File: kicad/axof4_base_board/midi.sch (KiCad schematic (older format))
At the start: 9 parts, among them J4 MIDI_IN, J5 MIDI_OUT, U8 6N137

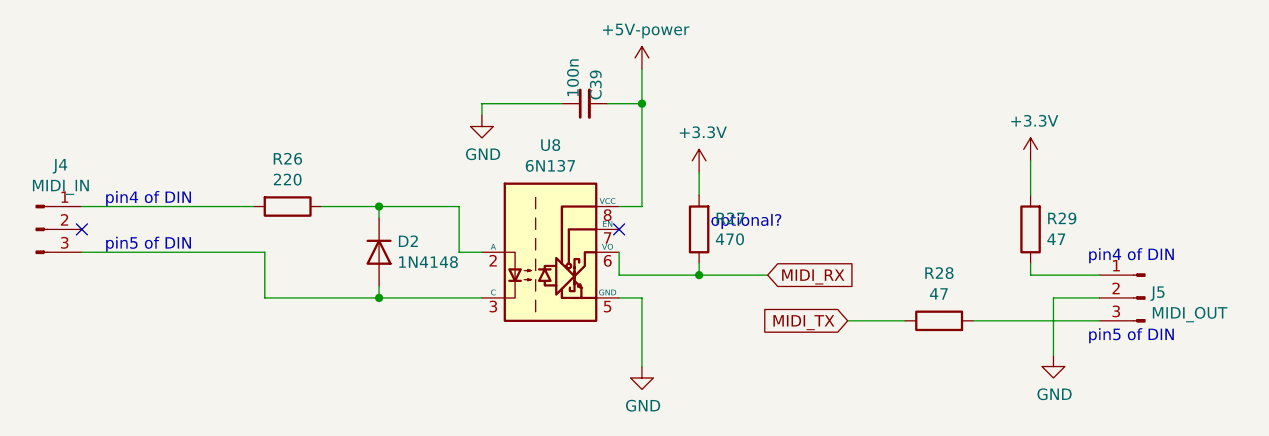
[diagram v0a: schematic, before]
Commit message: cleanup, dedicated PCB WIP
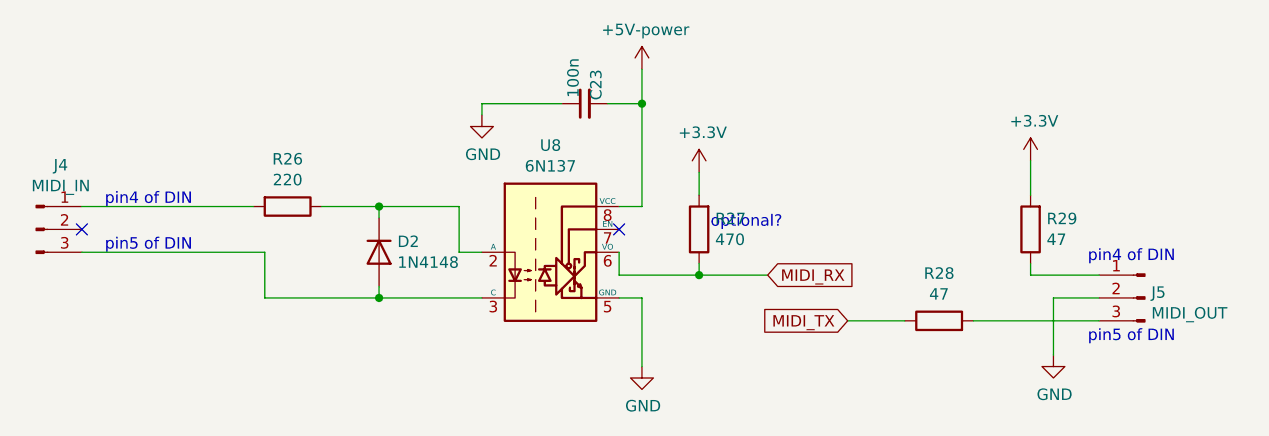
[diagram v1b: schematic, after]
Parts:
- J4, J5: footprint (none) -> Connector_PinHeader_2.54mm:PinHeader_1x03_P2.54mm_Vertical
- R26, R27, R28, R29: footprint (none) -> Resistor_SMD:R_1206_3216Metric_Pad1.42x1.75mm_HandSolder
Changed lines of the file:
@@
 $Descr A4 11693 8268
 encoding utf-8
-Sheet 6 6
+Sheet 6 7
 Title ""
 Date ""
@@
 AR Path="/5ED86ED4/5ECDCA2B" Ref="#PWR?"  Part="1"
 AR Path="/5EE2DB57/5ECDCA2B" Ref="#PWR037"  Part="1"
-F 0 "#PWR037" H 7800 3150 50  0001 C CNN
+AR Path="/5F736ED6/5ECDCA2B" Ref="#PWR?"  Part="1"
+F 0 "#PWR?" H 7800 3150 50  0001 C CNN
 F 1 "+3.3V" H 7815 3473 50  0000 C CNN
 F 2 "" H 7800 3300 50  0001 C CNN
@@
 AR Path="/5ED86ED4/5ECE0CFC" Ref="C?"  Part="1"
 AR Path="/5EE2DB57/5ECE0CFC" Ref="C39"  Part="1"
-F 0 "C39" H 6000 3000 50  0000 R CNN
+AR Path="/5F736ED6/5ECE0CFC" Ref="C?"  Part="1"
+F 0 "C?" H 6000 3000 50  0000 R CNN
 F 1 "100n" H 6050 3100 50  0000 R CNN
 F 2 "Capacitor_SMD:C_1206_3216Metric_Pad1.42x1.75mm_HandSolder" H 5850 3050 50  0001 C CNN
@@
 U 1 1 5EE31190
 P 4950 3700
-F 0 "D2" V 4904 3780 50  0000 L CNN
+AR Path="/5EE2DB57/5EE31190" Ref="D2"  Part="1"
+AR Path="/5F736ED6/5EE31190" Ref="D?"  Part="1"
+F 0 "D?" V 4904 3780 50  0000 L CNN
 F 1 "1N4148" V 4995 3780 50  0000 L CNN
 F 2 "Diode_THT:D_DO-35_SOD27_P7.62mm_Horizontal" H 4950 3525 50  0001 C CNN
@@
 U 1 1 5EE33166
 P 4550 3500
-F 0 "R26" V 4343 3500 50  0000 C CNN
+AR Path="/5EE2DB57/5EE33166" Ref="R26"  Part="1"
+AR Path="/5F736ED6/5EE33166" Ref="R?"  Part="1"
+F 0 "R?" V 4343 3500 50  0000 C CNN
 F 1 "220" V 4434 3500 50  0000 C CNN
-F 2 "" V 4480 3500 50  0001 C CNN
+F 2 "Resistor_SMD:R_1206_3216Metric_Pad1.42x1.75mm_HandSolder" V 4480 3500 50  0001 C CNN
 F 3 "~" H 4550 3500 50  0001 C CNN
 	1    4550 3500
@@
 U 1 1 5EE3734F
 P 3450 3600
-F 0 "J4" H 3558 3881 50  0000 C CNN
+AR Path="/5EE2DB57/5EE3734F" Ref="J4"  Part="1"
+AR Path="/5F736ED6/5EE3734F" Ref="J?"  Part="1"
+F 0 "J?" H 3558 3881 50  0000 C CNN
 F 1 "MIDI_IN" H 3558 3790 50  0000 C CNN
-F 2 "" H 3450 3600 50  0001 C CNN
+F 2 "Connector_PinHeader_2.54mm:PinHeader_1x03_P2.54mm_Vertical" H 3450 3600 50  0001 C CNN
 F 3 "~" H 3450 3600 50  0001 C CNN
 	1    3450 3600
@@
 U 1 1 5EE3A369
 P 6100 4200
-F 0 "#PWR036" H 6100 3950 50  0001 C CNN
+AR Path="/5EE2DB57/5EE3A369" Ref="#PWR036"  Part="1"
+AR Path="/5F736ED6/5EE3A369" Ref="#PWR?"  Part="1"
+F 0 "#PWR?" H 6100 3950 50  0001 C CNN
 F 1 "GND" H 6105 4027 50  0000 C CNN
 F 2 "" H 6100 4200 50  0001 C CNN
@@
 U 1 1 5EE3B250
 P 6350 3600
-F 0 "R27" H 6280 3554 50  0000 R CNN
+AR Path="/5EE2DB57/5EE3B250" Ref="R27"  Part="1"
+AR Path="/5F736ED6/5EE3B250" Ref="R?"  Part="1"
+F 0 "R?" H 6280 3554 50  0000 R CNN
 F 1 "470" H 6280 3645 50  0000 R CNN
-F 2 "" V 6280 3600 50  0001 C CNN
+F 2 "Resistor_SMD:R_1206_3216Metric_Pad1.42x1.75mm_HandSolder" V 6280 3600 50  0001 C CNN
 F 3 "~" H 6350 3600 50  0001 C CNN
 	1    6350 3600
@@
 U 1 1 5EE401BE
 P 5400 3100
-F 0 "#PWR034" H 5400 2850 50  0001 C CNN
+AR Path="/5EE2DB57/5EE401BE" Ref="#PWR034"  Part="1"
+AR Path="/5F736ED6/5EE401BE" Ref="#PWR?"  Part="1"
+F 0 "#PWR?" H 5400 2850 50  0001 C CNN
 F 1 "GND" H 5405 2927 50  0000 C CNN
 F 2 "" H 5400 3100 50  0001 C CNN
@@
 U 1 1 5EE4115F
 P 6100 2900
-F 0 "#PWR035" H 6100 2750 50  0001 C CNN
+AR Path="/5EE2DB57/5EE4115F" Ref="#PWR035"  Part="1"
+AR Path="/5F736ED6/5EE4115F" Ref="#PWR?"  Part="1"
+F 0 "#PWR?" H 6100 2750 50  0001 C CNN
 F 1 "+5V-power" H 6115 3073 50  0000 C CNN
 F 2 "" H 6100 2900 50  0001 C CNN
@@
 U 1 1 5EE45075
 P 7800 3600
-F 0 "R29" H 7730 3554 50  0000 R CNN
+AR Path="/5EE2DB57/5EE45075" Ref="R29"  Part="1"
+AR Path="/5F736ED6/5EE45075" Ref="R?"  Part="1"
+F 0 "R?" H 7730 3554 50  0000 R CNN
 F 1 "47" H 7730 3645 50  0000 R CNN
-F 2 "" V 7730 3600 50  0001 C CNN
+F 2 "Resistor_SMD:R_1206_3216Metric_Pad1.42x1.75mm_HandSolder" V 7730 3600 50  0001 C CNN
 F 3 "~" H 7800 3600 50  0001 C CNN
 	1    7800 3600
@@
 U 1 1 5EE46100
 P 8300 3900
-F 0 "J5" H 8272 3924 50  0000 R CNN
+AR Path="/5EE2DB57/5EE46100" Ref="J5"  Part="1"
+AR Path="/5F736ED6/5EE46100" Ref="J?"  Part="1"
+F 0 "J?" H 8272 3924 50  0000 R CNN
 F 1 "MIDI_OUT" H 8272 3833 50  0000 R CNN
-F 2 "" H 8300 3900 50  0001 C CNN
+F 2 "Connector_PinHeader_2.54mm:PinHeader_1x03_P2.54mm_Vertical" H 8300 3900 50  0001 C CNN
 F 3 "~" H 8300 3900 50  0001 C CNN
 	1    8300 3900
@@
 U 1 1 5EE499CC
 P 7400 4000
-F 0 "R28" V 7607 4000 50  0000 C CNN
+AR Path="/5EE2DB57/5EE499CC" Ref="R28"  Part="1"
+AR Path="/5F736ED6/5EE499CC" Ref="R?"  Part="1"
+F 0 "R?" V 7607 4000 50  0000 C CNN
 F 1 "47" V 7516 4000 50  0000 C CNN
-F 2 "" V 7330 4000 50  0001 C CNN
+F 2 "Resistor_SMD:R_1206_3216Metric_Pad1.42x1.75mm_HandSolder" V 7330 4000 50  0001 C CNN
 F 3 "~" H 7400 4000 50  0001 C CNN
 	1    7400 4000
@@
 U 1 1 5EE4E2E6
 P 7900 4150
-F 0 "#PWR038" H 7900 3900 50  0001 C CNN
+AR Path="/5EE2DB57/5EE4E2E6" Ref="#PWR038"  Part="1"
+AR Path="/5F736ED6/5EE4E2E6" Ref="#PWR?"  Part="1"
+F 0 "#PWR?" H 7900 3900 50  0001 C CNN
 F 1 "GND" H 7905 3977 50  0000 C CNN
 F 2 "" H 7900 4150 50  0001 C CNN
@@
 U 1 1 5EE5AB46
 P 5700 3700
-F 0 "U8" H 5700 4167 50  0000 C CNN
+AR Path="/5EE2DB57/5EE5AB46" Ref="U8"  Part="1"
+AR Path="/5F736ED6/5EE5AB46" Ref="U?"  Part="1"
+F 0 "U?" H 5700 4167 50  0000 C CNN
 F 1 "6N137" H 5700 4076 50  0000 C CNN
 F 2 "Package_DIP:DIP-8_W7.62mm" H 5700 3200 50  0001 C CNN
@@
 AR Path="/5ED86ED4/5EE65032" Ref="#PWR?"  Part="1"
 AR Path="/5EE2DB57/5EE65032" Ref="#PWR039"  Part="1"
-F 0 "#PWR039" H 6350 3200 50  0001 C CNN
+AR Path="/5F736ED6/5EE65032" Ref="#PWR?"  Part="1"
+F 0 "#PWR?" H 6350 3200 50  0001 C CNN
 F 1 "+3.3V" H 6365 3523 50  0000 C CNN
 F 2 "" H 6350 3350 50  0001 C CNN

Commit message: kicad pcb backup, hohum axoctrl study
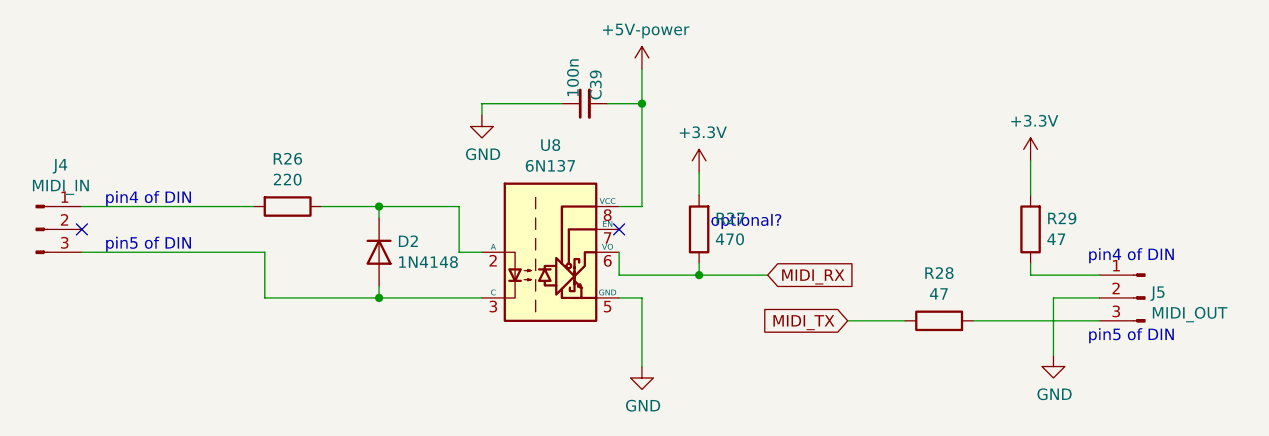
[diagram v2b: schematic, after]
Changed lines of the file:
@@
 AR Path="/5EE2DB57/5ECDCA2B" Ref="#PWR037"  Part="1"
 AR Path="/5F736ED6/5ECDCA2B" Ref="#PWR?"  Part="1"
-F 0 "#PWR?" H 7800 3150 50  0001 C CNN
+F 0 "#PWR037" H 7800 3150 50  0001 C CNN
 F 1 "+3.3V" H 7815 3473 50  0000 C CNN
 F 2 "" H 7800 3300 50  0001 C CNN
@@
 AR Path="/5EE2DB57/5ECE0CFC" Ref="C39"  Part="1"
 AR Path="/5F736ED6/5ECE0CFC" Ref="C?"  Part="1"
-F 0 "C?" H 6000 3000 50  0000 R CNN
+F 0 "C39" H 6000 3000 50  0000 R CNN
 F 1 "100n" H 6050 3100 50  0000 R CNN
 F 2 "Capacitor_SMD:C_1206_3216Metric_Pad1.42x1.75mm_HandSolder" H 5850 3050 50  0001 C CNN
@@
 AR Path="/5EE2DB57/5EE31190" Ref="D2"  Part="1"
 AR Path="/5F736ED6/5EE31190" Ref="D?"  Part="1"
-F 0 "D?" V 4904 3780 50  0000 L CNN
+F 0 "D2" V 4904 3780 50  0000 L CNN
 F 1 "1N4148" V 4995 3780 50  0000 L CNN
 F 2 "Diode_THT:D_DO-35_SOD27_P7.62mm_Horizontal" H 4950 3525 50  0001 C CNN
@@
 AR Path="/5EE2DB57/5EE33166" Ref="R26"  Part="1"
 AR Path="/5F736ED6/5EE33166" Ref="R?"  Part="1"
-F 0 "R?" V 4343 3500 50  0000 C CNN
+F 0 "R26" V 4343 3500 50  0000 C CNN
 F 1 "220" V 4434 3500 50  0000 C CNN
 F 2 "Resistor_SMD:R_1206_3216Metric_Pad1.42x1.75mm_HandSolder" V 4480 3500 50  0001 C CNN
@@
 AR Path="/5EE2DB57/5EE3734F" Ref="J4"  Part="1"
 AR Path="/5F736ED6/5EE3734F" Ref="J?"  Part="1"
-F 0 "J?" H 3558 3881 50  0000 C CNN
+F 0 "J4" H 3558 3881 50  0000 C CNN
 F 1 "MIDI_IN" H 3558 3790 50  0000 C CNN
 F 2 "Connector_PinHeader_2.54mm:PinHeader_1x03_P2.54mm_Vertical" H 3450 3600 50  0001 C CNN
@@
 AR Path="/5EE2DB57/5EE3A369" Ref="#PWR036"  Part="1"
 AR Path="/5F736ED6/5EE3A369" Ref="#PWR?"  Part="1"
-F 0 "#PWR?" H 6100 3950 50  0001 C CNN
+F 0 "#PWR036" H 6100 3950 50  0001 C CNN
 F 1 "GND" H 6105 4027 50  0000 C CNN
 F 2 "" H 6100 4200 50  0001 C CNN
@@
 AR Path="/5EE2DB57/5EE3B250" Ref="R27"  Part="1"
 AR Path="/5F736ED6/5EE3B250" Ref="R?"  Part="1"
-F 0 "R?" H 6280 3554 50  0000 R CNN
+F 0 "R27" H 6280 3554 50  0000 R CNN
 F 1 "470" H 6280 3645 50  0000 R CNN
 F 2 "Resistor_SMD:R_1206_3216Metric_Pad1.42x1.75mm_HandSolder" V 6280 3600 50  0001 C CNN
@@
 AR Path="/5EE2DB57/5EE401BE" Ref="#PWR034"  Part="1"
 AR Path="/5F736ED6/5EE401BE" Ref="#PWR?"  Part="1"
-F 0 "#PWR?" H 5400 2850 50  0001 C CNN
+F 0 "#PWR034" H 5400 2850 50  0001 C CNN
 F 1 "GND" H 5405 2927 50  0000 C CNN
 F 2 "" H 5400 3100 50  0001 C CNN
@@
 AR Path="/5EE2DB57/5EE4115F" Ref="#PWR035"  Part="1"
 AR Path="/5F736ED6/5EE4115F" Ref="#PWR?"  Part="1"
-F 0 "#PWR?" H 6100 2750 50  0001 C CNN
+F 0 "#PWR035" H 6100 2750 50  0001 C CNN
 F 1 "+5V-power" H 6115 3073 50  0000 C CNN
 F 2 "" H 6100 2900 50  0001 C CNN
@@
 AR Path="/5EE2DB57/5EE45075" Ref="R29"  Part="1"
 AR Path="/5F736ED6/5EE45075" Ref="R?"  Part="1"
-F 0 "R?" H 7730 3554 50  0000 R CNN
+F 0 "R29" H 7730 3554 50  0000 R CNN
 F 1 "47" H 7730 3645 50  0000 R CNN
 F 2 "Resistor_SMD:R_1206_3216Metric_Pad1.42x1.75mm_HandSolder" V 7730 3600 50  0001 C CNN
@@
 AR Path="/5EE2DB57/5EE46100" Ref="J5"  Part="1"
 AR Path="/5F736ED6/5EE46100" Ref="J?"  Part="1"
-F 0 "J?" H 8272 3924 50  0000 R CNN
+F 0 "J5" H 8272 3924 50  0000 R CNN
 F 1 "MIDI_OUT" H 8272 3833 50  0000 R CNN
 F 2 "Connector_PinHeader_2.54mm:PinHeader_1x03_P2.54mm_Vertical" H 8300 3900 50  0001 C CNN
@@
 AR Path="/5EE2DB57/5EE499CC" Ref="R28"  Part="1"
 AR Path="/5F736ED6/5EE499CC" Ref="R?"  Part="1"
-F 0 "R?" V 7607 4000 50  0000 C CNN
+F 0 "R28" V 7607 4000 50  0000 C CNN
 F 1 "47" V 7516 4000 50  0000 C CNN
 F 2 "Resistor_SMD:R_1206_3216Metric_Pad1.42x1.75mm_HandSolder" V 7330 4000 50  0001 C CNN
@@
 AR Path="/5EE2DB57/5EE4E2E6" Ref="#PWR038"  Part="1"
 AR Path="/5F736ED6/5EE4E2E6" Ref="#PWR?"  Part="1"
-F 0 "#PWR?" H 7900 3900 50  0001 C CNN
+F 0 "#PWR038" H 7900 3900 50  0001 C CNN
 F 1 "GND" H 7905 3977 50  0000 C CNN
 F 2 "" H 7900 4150 50  0001 C CNN
@@
 AR Path="/5EE2DB57/5EE5AB46" Ref="U8"  Part="1"
 AR Path="/5F736ED6/5EE5AB46" Ref="U?"  Part="1"
-F 0 "U?" H 5700 4167 50  0000 C CNN
+F 0 "U8" H 5700 4167 50  0000 C CNN
 F 1 "6N137" H 5700 4076 50  0000 C CNN
 F 2 "Package_DIP:DIP-8_W7.62mm" H 5700 3200 50  0001 C CNN
@@
 AR Path="/5EE2DB57/5EE65032" Ref="#PWR039"  Part="1"
 AR Path="/5F736ED6/5EE65032" Ref="#PWR?"  Part="1"
-F 0 "#PWR?" H 6350 3200 50  0001 C CNN
+F 0 "#PWR039" H 6350 3200 50  0001 C CNN
 F 1 "+3.3V" H 6365 3523 50  0000 C CNN
 F 2 "" H 6350 3350 50  0001 C CNN

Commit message: rollback kicad project to use STM32F4DISCOVERY
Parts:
- C23: footprint Capacitor_SMD:C_1206_3216Metric_Pad1.42x1.75mm_HandSolder -> Capacitor_SMD:C_0603_1608Metric
- D2: footprint Diode_THT:D_DO-35_SOD27_P7.62mm_Horizontal -> Diode_SMD:D_SOD-123
- R26, R27, R28, R29: footprint Resistor_SMD:R_1206_3216Metric_Pad1.42x1.75mm_HandSolder -> Resistor_SMD:R_0603_1608Metric
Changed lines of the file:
@@
 F 0 "C39" H 6000 3000 50  0000 R CNN
 F 1 "100n" H 6050 3100 50  0000 R CNN
-F 2 "Capacitor_SMD:C_1206_3216Metric_Pad1.42x1.75mm_HandSolder" H 5850 3050 50  0001 C CNN
+F 2 "Capacitor_SMD:C_0603_1608Metric" H 5850 3050 50  0001 C CNN
 F 3 "~" H 5850 3050 50  0001 C CNN
 	1    5850 3050
@@
 F 0 "D2" V 4904 3780 50  0000 L CNN
 F 1 "1N4148" V 4995 3780 50  0000 L CNN
-F 2 "Diode_THT:D_DO-35_SOD27_P7.62mm_Horizontal" H 4950 3525 50  0001 C CNN
+F 2 "Diode_SMD:D_SOD-123" H 4950 3525 50  0001 C CNN
 F 3 "https://assets.nexperia.com/documents/data-sheet/1N4148_1N4448.pdf" H 4950 3700 50  0001 C CNN
 	1    4950 3700
@@
 F 0 "R26" V 4343 3500 50  0000 C CNN
 F 1 "220" V 4434 3500 50  0000 C CNN
-F 2 "Resistor_SMD:R_1206_3216Metric_Pad1.42x1.75mm_HandSolder" V 4480 3500 50  0001 C CNN
+F 2 "Resistor_SMD:R_0603_1608Metric" V 4480 3500 50  0001 C CNN
 F 3 "~" H 4550 3500 50  0001 C CNN
 	1    4550 3500
@@
 F 0 "R27" H 6280 3554 50  0000 R CNN
 F 1 "470" H 6280 3645 50  0000 R CNN
-F 2 "Resistor_SMD:R_1206_3216Metric_Pad1.42x1.75mm_HandSolder" V 6280 3600 50  0001 C CNN
+F 2 "Resistor_SMD:R_0603_1608Metric" V 6280 3600 50  0001 C CNN
 F 3 "~" H 6350 3600 50  0001 C CNN
 	1    6350 3600
@@
 F 0 "R29" H 7730 3554 50  0000 R CNN
 F 1 "47" H 7730 3645 50  0000 R CNN
-F 2 "Resistor_SMD:R_1206_3216Metric_Pad1.42x1.75mm_HandSolder" V 7730 3600 50  0001 C CNN
+F 2 "Resistor_SMD:R_0603_1608Metric" V 7730 3600 50  0001 C CNN
 F 3 "~" H 7800 3600 50  0001 C CNN
 	1    7800 3600
@@
 F 0 "R28" V 7607 4000 50  0000 C CNN
 F 1 "47" V 7516 4000 50  0000 C CNN
-F 2 "Resistor_SMD:R_1206_3216Metric_Pad1.42x1.75mm_HandSolder" V 7330 4000 50  0001 C CNN
+F 2 "Resistor_SMD:R_0603_1608Metric" V 7330 4000 50  0001 C CNN
 F 3 "~" H 7400 4000 50  0001 C CNN
 	1    7400 4000
@@
 Text Notes 8050 3750 0    50   ~ 0
 pin4 of DIN
-$Comp
-L Isolator:6N137 U8
-U 1 1 5EE5AB46
-P 5700 3700
-AR Path="/5EE2DB57/5EE5AB46" Ref="U8"  Part="1"
-AR Path="/5F736ED6/5EE5AB46" Ref="U?"  Part="1"
-F 0 "U8" H 5700 4167 50  0000 C CNN
-F 1 "6N137" H 5700 4076 50  0000 C CNN
-F 2 "Package_DIP:DIP-8_W7.62mm" H 5700 3200 50  0001 C CNN
-F 3 "https://docs.broadcom.com/docs/AV02-0940EN" H 4850 4250 50  0001 C CNN
-	1    5700 3700
-	1    0    0    -1
-$EndComp
 Wire Wire Line
 	6000 3800 6000 3700
@@
 Wire Wire Line
 	6350 3350 6350 3450
+$Comp
+L Isolator:6N137 U8
+U 1 1 5EE5AB46
+P 5700 3700
+AR Path="/5EE2DB57/5EE5AB46" Ref="U8"  Part="1"
+AR Path="/5F736ED6/5EE5AB46" Ref="U?"  Part="1"
+F 0 "U8" H 5700 4167 50  0000 C CNN
+F 1 "6N137" H 5700 4076 50  0000 C CNN
+F 2 "Package_DIP:DIP-8_W7.62mm" H 5700 3200 50  0001 C CNN
+F 3 "https://docs.broadcom.com/docs/AV02-0940EN" H 4850 4250 50  0001 C CNN
+	1    5700 3700
+	1    0    0    -1
+$EndComp
 $EndSCHEMATC
